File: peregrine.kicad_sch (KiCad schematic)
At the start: 49 parts, among them J1 Barrel_Jack, J2 Ext., J3 Ext., J4 50Ω, SW1 SW_SPDT, SW2 SW_SPDT, U1 MIC5365-3.3YD5, U2 MIC5365-3.3YD5, U3 4020, U4 TS5A3159ADBVR, U5 74AUC1G86, U6 74AUC2G34, X1 ASV-16MHz

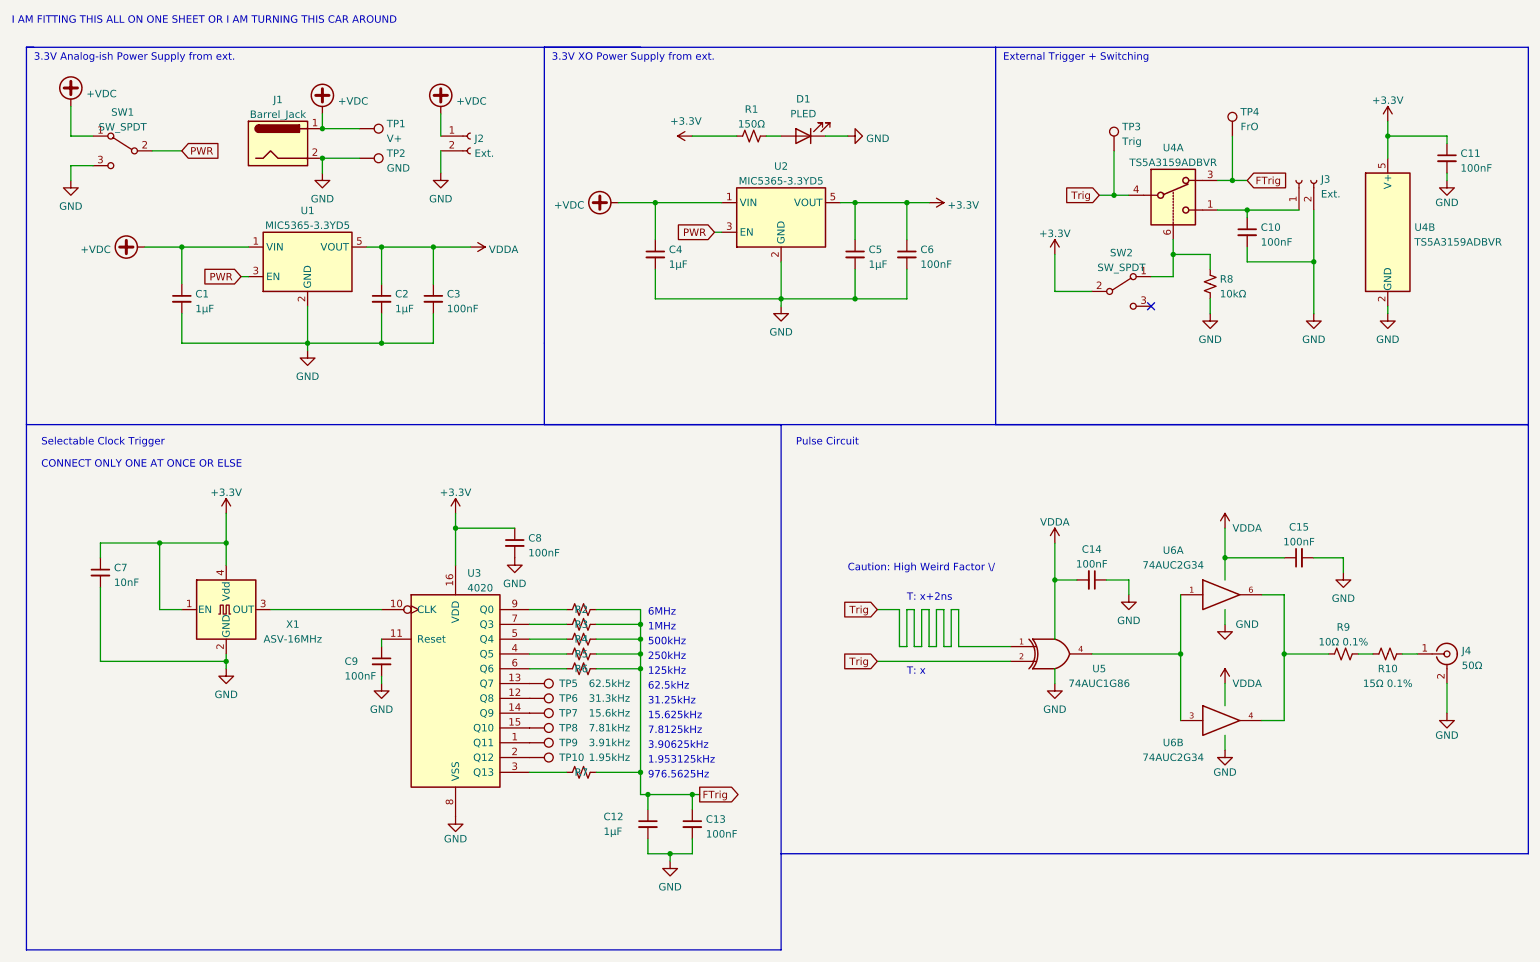
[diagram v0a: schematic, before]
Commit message: redesign
why yes i redesigned half of the entire board
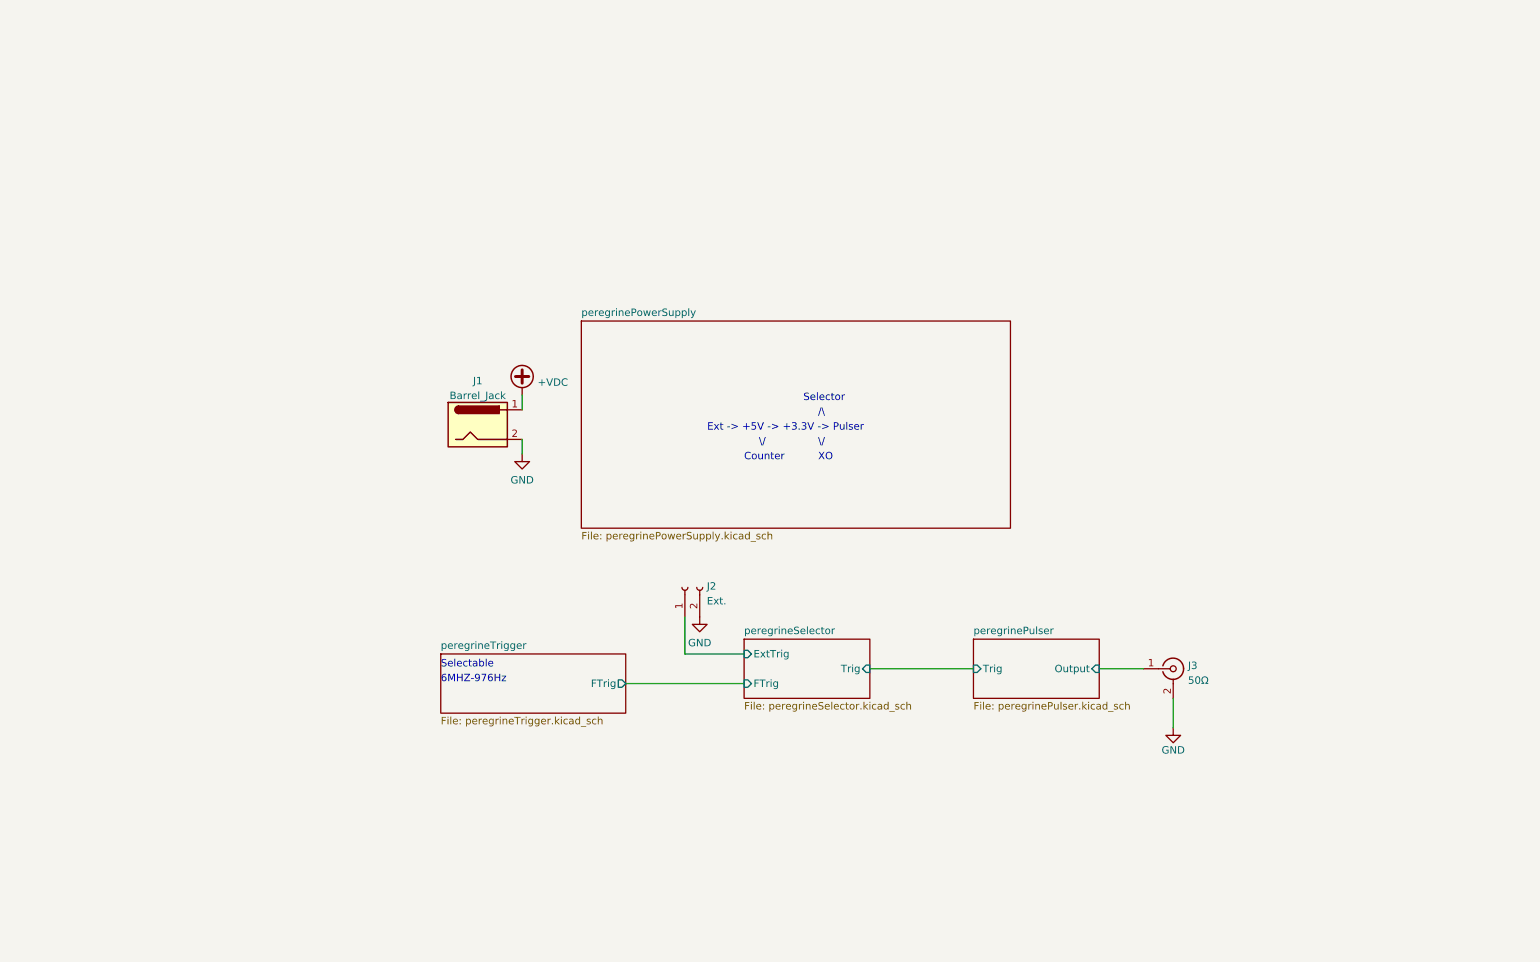
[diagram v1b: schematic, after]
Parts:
- removed C1, C12, C2, C4, C5: 1μF, Capacitor_SMD:C_0603_1608Metric_Pad1.08x0.95mm_HandSolder, symbol Device:C_Small
- removed C10, C11, C13, C14, C15, C3, C6, C8, C9: 100nF, Capacitor_SMD:C_0603_1608Metric_Pad1.08x0.95mm_HandSolder, symbol Device:C_Small
- removed C7: 10nF, Capacitor_SMD:C_0603_1608Metric_Pad1.08x0.95mm_HandSolder, symbol Device:C_Small
- removed D1: PLED, LED_SMD:LED_0603_1608Metric_Pad1.05x0.95mm_HandSolder, symbol Device:LED
- removed J3: Ext., Connector_PinHeader_2.54mm:PinHeader_1x02_P2.54mm_Vertical, symbol Connector:Conn_01x02_Female
- removed J4: 50Ω, CONSMA020:LINX_CONSMA020.062-G, symbol Connector:Conn_Coaxial
- removed R1: 150Ω, Resistor_SMD:R_0603_1608Metric_Pad0.98x0.95mm_HandSolder, symbol Device:R_Small_US
- removed R10: 15Ω 0.1%, Resistor_SMD:R_0603_1608Metric_Pad0.98x0.95mm_HandSolder, symbol Device:R_Small_US
- removed R2, R3, R4, R5, R6, R7: 0, Resistor_SMD:R_0402_1005Metric_Pad0.72x0.64mm_HandSolder, symbol Device:R_Small_US
- removed R8: 10kΩ, Resistor_SMD:R_0603_1608Metric_Pad0.98x0.95mm_HandSolder, symbol Device:R_Small_US
- removed R9: 10Ω 0.1%, Resistor_SMD:R_0603_1608Metric_Pad0.98x0.95mm_HandSolder, symbol Device:R_Small_US
- removed SW1, SW2: SW_SPDT, ul_JS102011SCQN:JS102011SCQN, symbol Switch:SW_SPDT
- removed TP1: V+, TestPoint:TestPoint_Pad_1.5x1.5mm, symbol Connector:TestPoint
- removed TP10: 1.95kHz, TestPoint:TestPoint_Pad_D1.0mm, symbol Connector:TestPoint
- removed TP2: GND, TestPoint:TestPoint_Pad_1.5x1.5mm, symbol Connector:TestPoint
- removed TP3: Trig, TestPoint:TestPoint_Pad_D1.0mm, symbol Connector:TestPoint
- removed TP4: FrO, TestPoint:TestPoint_Pad_D1.0mm, symbol Connector:TestPoint
- removed TP5: 62.5kHz, TestPoint:TestPoint_Pad_D1.0mm, symbol Connector:TestPoint
- removed TP6: 31.3kHz, TestPoint:TestPoint_Pad_D1.0mm, symbol Connector:TestPoint
- removed TP7: 15.6kHz, TestPoint:TestPoint_Pad_D1.0mm, symbol Connector:TestPoint
- removed TP8: 7.81kHz, TestPoint:TestPoint_Pad_D1.0mm, symbol Connector:TestPoint
- removed TP9: 3.91kHz, TestPoint:TestPoint_Pad_D1.0mm, symbol Connector:TestPoint
- removed U1, U2: MIC5365-3.3YD5, Package_TO_SOT_SMD:SOT-23-5_HandSoldering, symbol Regulator_Linear:MIC5365-3.3YD5
- removed U3: 4020, Package_SO:TSSOP-16_4.4x5mm_P0.65mm, symbol 4xxx:4020
- removed U4: TS5A3159ADBVR, Package_TO_SOT_SMD:SOT-23-6_Handsoldering, symbol Analog_Switch:TS5A3159ADBVR
- removed U5: 74AUC1G86, Package_TO_SOT_SMD:SOT-353_SC-70-5_Handsoldering, symbol 74xGxx:74AUC1G86
- removed U6: 74AUC2G34, Package_TO_SOT_SMD:SOT-363_SC-70-6_Handsoldering, symbol 74xGxx:74AUC2G34
- removed X1: ASV-16MHz, Oscillator:Oscillator_SMD_Abracon_ASV-4Pin_7.0x5.1mm, symbol Oscillator:ASV-xxxMHz
- added J3: 50Ω, CONSMA020:LINX_CONSMA020.062-G, symbol Connector:Conn_Coaxial
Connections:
- net +VDC: no longer J2.1 (Pin_1)
- net GND: now also J3.2 (Ext)
- new net peregrinePulser/Output: J3.1 (In)
- new net peregrineSelector/ExtTrig: J2.1 (Pin_1)
- no-connect marks 1 -> 0
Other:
- added sheet peregrinePowerSupply (peregrinePowerSupply.kicad_sch)
- added sheet peregrinePulser (peregrinePulser.kicad_sch)
- added sheet peregrineSelector (peregrineSelector.kicad_sch)
- added sheet peregrineTrigger (peregrineTrigger.kicad_sch)
- note added: "/\"
- note added: "6MHZ-976Hz"
- note added: "Counter"
- note added: "Ext -> +5V -> +3.3V -> Pulser"
- note added: "Selectable"
- note added: "Selector"
- note added: "XO"
- note added: "\/"
- note removed: "1.953125kHz"
- note removed: "125kHz"
- note removed: "15.625kHz"
- note removed: "1MHz"
- note removed: "250kHz"
- note removed: "3.3V Analog-ish Power Supply from ext."
- note removed: "3.3V XO Power Supply from ext."
- note removed: "3.90625kHz"
- note removed: "31.25kHz"
- note removed: "500kHz"
- note removed: "62.5kHz"
- note removed: "6MHz"
- note removed: "7.8125kHz"
- note removed: "976.5625Hz"
- note removed: "CONNECT ONLY ONE AT ONCE OR ELSE"
- note removed: "Caution: High Weird Factor \/"
- note removed: "External Trigger + Switching"
- note removed: "I AM FITTING THIS ALL ON ONE SHEET OR I AM TURNING THIS CAR AROUND"
- note removed: "Pulse Circuit"
- note removed: "Selectable Clock Trigger"
- note removed: "T: x"
- note removed: "T: x+2ns"
